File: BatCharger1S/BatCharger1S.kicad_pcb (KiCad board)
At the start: 2 copper layers, 53.7 x 25.7 mm, 58 parts, among them J1 USB_C_Receptacle, J2 01x02, J3 01x02, J4 01x02, J5 01x02, J6 Conn_01x03, J7 01x02, Q1 Si2323DS, Q2 Si2323DS, Q3 Si2323DS, Q4 Si2323DS, U1 USBLC6-2P6, U2 MAX17048G+T10, U3 MCP73833-AMI/UN, U4 TLV75533PDBV

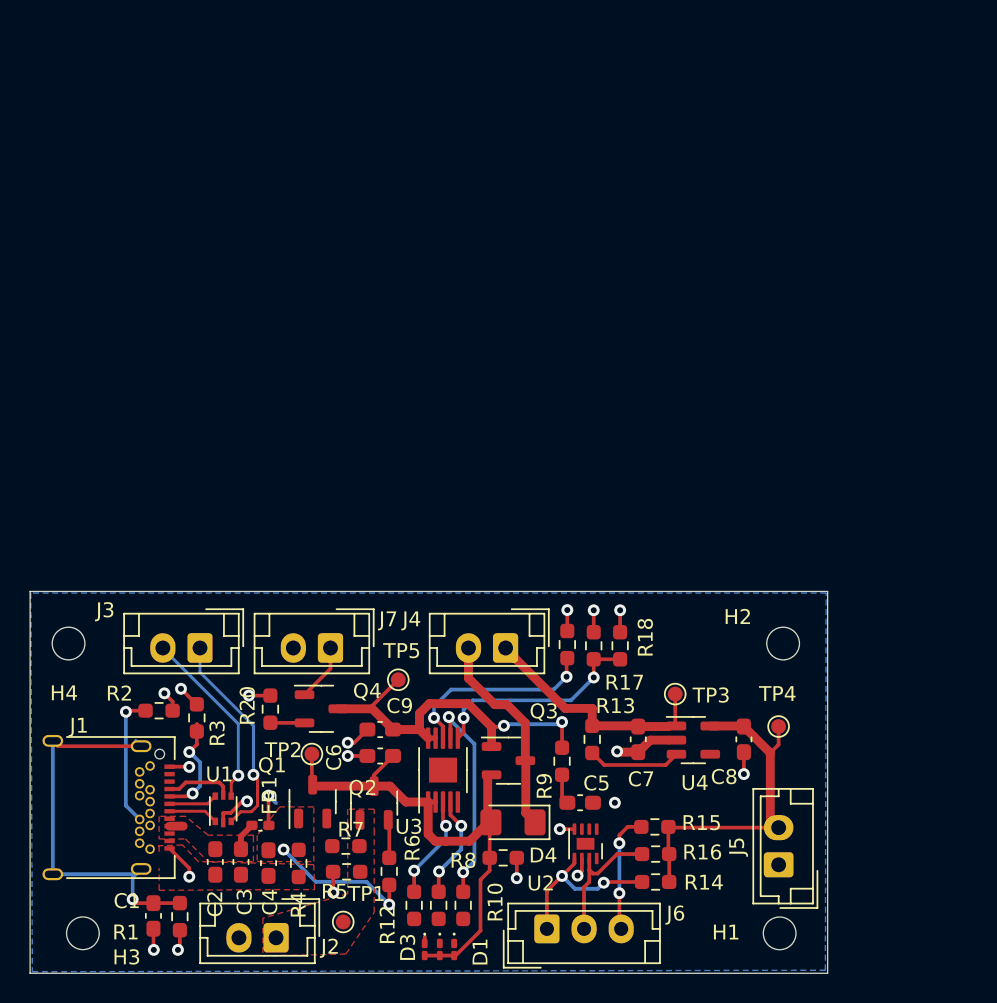
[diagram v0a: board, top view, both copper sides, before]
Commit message: v2Layout
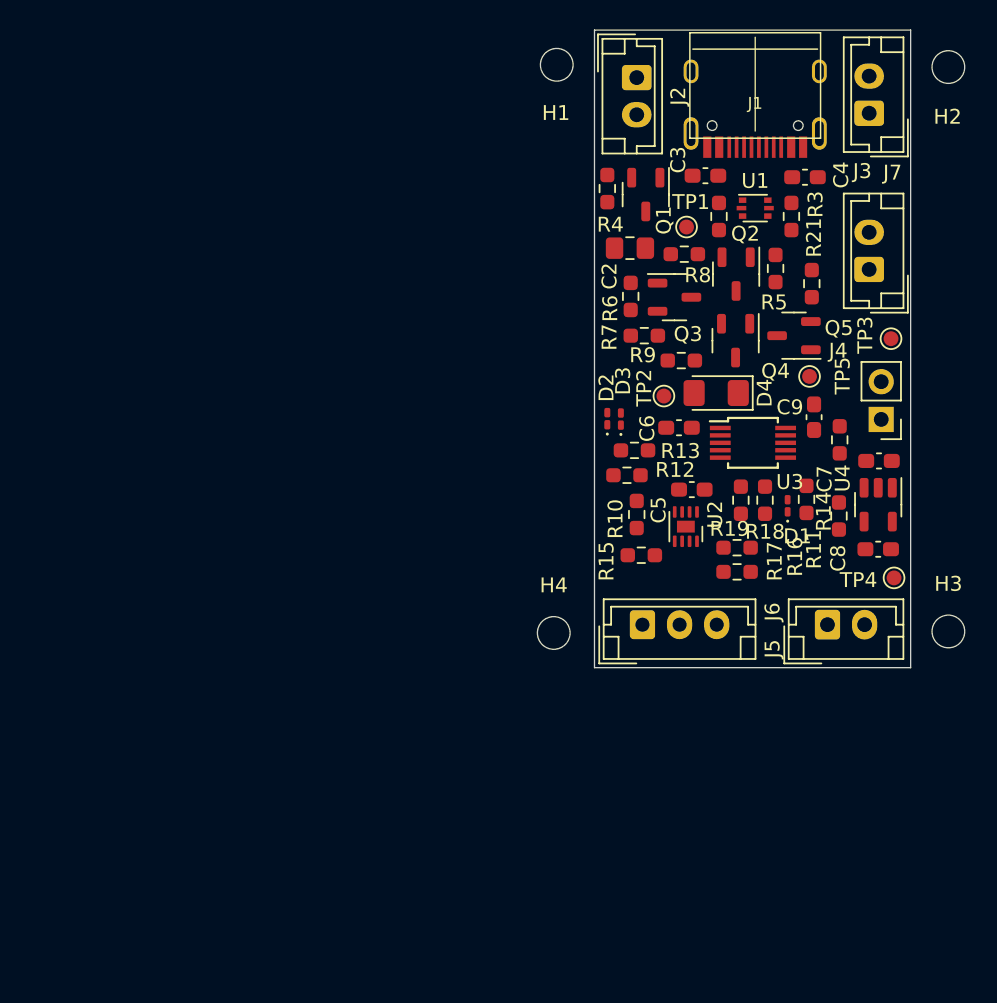
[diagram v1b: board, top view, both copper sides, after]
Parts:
- removed C1: 10u, Capacitor_SMD:C_0603_1608Metric_Pad1.08x0.95mm_HandSolder
- removed FB1: 100 @ 100MHz, Inductor_SMD:L_0402_1005Metric_Pad0.77x0.64mm_HandSolder
- removed R1: 1M, Resistor_SMD:R_0603_1608Metric_Pad0.98x0.95mm_HandSolder
- added Q5: Si2323DS, Package_TO_SOT_SMD:SOT-23-3, F.Cu at (145.6, 64.2)
- added R21: 100k, Resistor_SMD:R_0603_1608Metric_Pad0.98x0.95mm_HandSolder, F.Cu at (146.8, 60.7)
- C2: footprint Capacitor_SMD:C_0603_1608Metric_Pad1.08x0.95mm_HandSolder -> Capacitor_SMD:C_0805_2012Metric_Pad1.18x1.45mm_HandSolder
- C3: value 1u -> 10u
- J1: value USB_C_Receptacle -> TYPE-C-31-M-12; footprint Connector_USB:USB_C_Receptacle_Amphenol_12401548E4-2A -> Connector_USB:TYPE-C-31-M-12
- J4: footprint Connector_JST:JST_EH_B2B-EH-A_1x02_P2.50mm_Vertical -> Connector_PinHeader_2.54mm:PinHeader_1x02_P2.54mm_Vertical
- J5: value 01x02 -> Conn_01x03; footprint Connector_JST:JST_EH_B2B-EH-A_1x02_P2.50mm_Vertical -> Connector_JST:JST_EH_B3B-EH-A_1x03_P2.50mm_Vertical
- J6: value Conn_01x03 -> 01x02; footprint Connector_JST:JST_EH_B3B-EH-A_1x03_P2.50mm_Vertical -> Connector_JST:JST_EH_B2B-EH-A_1x02_P2.50mm_Vertical
- R10: value 1k -> 0R
- R13: value 100k -> 1k
- R14, R6: value 10k -> 100k
- R15: value 2k2 -> 10k
- R17: value 1k -> 2k2
- R19: value 10k -> 1k
- R20, R4, R8: value 100k -> 10k
- R9: value 0R -> 100k
- U3: footprint Package_SO:MSOP-10-1EP_3x3mm_P0.5mm_EP1.68x1.88mm -> Package_SO:MSOP-10_3x3mm_P0.5mm
- moved J1 66.6 mm to (143.0, 46.4), turned to 180 degrees
- moved J2 62.8 mm to (135.0, 46.8), turned to -90 degrees
- moved H3 61.7 mm to (156.0, 84.1)
- moved H1 60.4 mm to (129.6, 45.9)
- moved C4 58.6 mm to (146.4, 53.5), turned to 0 degrees
- moved J3 57.7 mm to (150.7, 49.2), turned to 90 degrees
- moved C3 55.8 mm to (139.7, 53.4), turned to 180 degrees
- moved U1 54.0 mm to (143.0, 55.6), turned to 0 degrees
- moved R3 52.4 mm to (145.4, 56.1), turned to -90 degrees
- moved TP1 52.2 mm to (138.4, 56.8)
- moved R2 50.3 mm to (140.6, 56.1), turned to -90 degrees
- moved R4 50.0 mm to (133.0, 54.3)
- moved C2 49.9 mm to (134.6, 58.3), turned to 180 degrees
- moved R5 49.8 mm to (144.4, 59.6), turned to -90 degrees
- moved Q1 46.6 mm to (135.6, 54.7), turned to -90 degrees
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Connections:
- C2 pad 1: /VBUS_IN -> +5V
- C3 pad 1: /VBUS_IN -> VBUS
- J1 pad A4: /VBUS_IN -> VBUS
- J1 pad A8: unconnected-(J1-SBU1-PadA8) -> (no net)
- J1 pad A9: /VBUS_IN -> VBUS
- J1 pad B4: /VBUS_IN -> VBUS
- J1 pad B6: /CON_USB_P -> (no net)
- J1 pad B7: /CON_USB_N -> (no net)
- J1 pad B8: unconnected-(J1-SBU2-PadB8) -> (no net)
- J1 pad B9: /VBUS_IN -> VBUS
- J1 pad S1: Net-(J1-SHIELD) -> GND
- J2 pad 1: +5V -> GND
- J2 pad 2: GND -> Net-(J2-Pin_2)
- J5 pad 1: GND -> /Alert
- J5 pad 2: +3V3 -> /SDA
- J6 pad 1: /Alert -> GND
- J6 pad 2: /SCl -> +3V3
- Q1 pad 1: VBUS -> Net-(J2-Pin_2)
- Q1 pad 3: VDC -> +5V
- Q2 pad 1: +5V -> VBUS
- Q3 pad 1: +BATT -> +5V
- Q3 pad 2: VDC -> Net-(Q3-G)
- Q3 pad 3: /pwrSwitch -> VDC
- Q4 pad 1: Net-(J7-Pin_1) -> +BATT
- Q4 pad 2: Net-(Q4-G) -> VDC
- Q4 pad 3: +BATT -> /pwrSwitch
- R10 pad 1: Net-(D1-K) -> +BATT
- R10 pad 2: Net-(U3-nPG) -> /vBatSense
- R11 pad 1: Net-(D2-K) -> Net-(D1-K)
- R11 pad 2: Net-(U3-STAT2) -> Net-(U3-nPG)
- R12 pad 1: Net-(D3-K) -> Net-(D2-K)
- R12 pad 2: Net-(U3-STAT1) -> Net-(U3-STAT2)
- R13 pad 1: VCC -> Net-(D3-K)
- R13 pad 2: Net-(U4-EN) -> Net-(U3-STAT1)
- R14 pad 1: +3V3 -> VCC
- R14 pad 2: /Alert -> Net-(U4-EN)
- R15 pad 2: /SDA -> /Alert
- R16 pad 2: /SCl -> /SDA
- R17 pad 1: Net-(U3-PROG) -> +3V3
- R17 pad 2: GND -> /SCl
- R19 pad 1: Net-(U3-THERM) -> Net-(U3-PROG)
- R20 pad 1: GND -> Net-(U3-THERM)
- R20 pad 2: Net-(Q4-G) -> GND
- R4 pad 1: VBUS -> Net-(Q1-G)
- R5 pad 1: GND -> VBUS
- R5 pad 2: +5V -> GND
- R6 pad 1: VBUS -> GND
- R6 pad 2: Net-(Q2-G) -> +5V
- R7 pad 1: Net-(Q1-G) -> VBUS
- R7 pad 2: +5V -> Net-(Q3-G)
- R8 pad 1: GND -> Net-(Q2-G)
- R8 pad 2: VDC -> +5V
- R9 pad 1: +BATT -> GND
- R9 pad 2: /vBatSense -> VDC
- U1 pad 5: /VBUS_IN -> VBUS
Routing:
- net VDC: track 36.0 -> 0.00 mm
- net GND: track 31.1 -> 0.00 mm, vias 20 -> 0
- net Net-(J1-SHIELD): track 26.7 -> 0.00 mm, vias 1 -> 0
- net +BATT: track 25.2 -> 0.00 mm, vias 2 -> 0
- net +3V3: track 23.5 -> 0.00 mm
- net VCC: track 16.0 -> 0.00 mm
- net Net-(U3-PROG): track 14.8 -> 0.00 mm, vias 2 -> 0
- net /USB_N: track 14.3 -> 0.00 mm, vias 1 -> 0
- net Net-(U3-nPG): track 14.3 -> 0.00 mm, vias 2 -> 0
- net /pwrSwitch: track 14.3 -> 0.00 mm
- net Net-(U3-THERM): track 13.6 -> 0.00 mm, vias 2 -> 0
- net VBUS: track 12.8 -> 0.00 mm, vias 3 -> 0
- net /USB_P: track 12.2 -> 0.00 mm, vias 1 -> 0
- net /Alert: track 11.4 -> 0.00 mm, vias 2 -> 0
- net /SCl: track 9.83 -> 0.00 mm
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- removed copper zone on F.Cu, net +5V
- removed copper zone on F.Cu, net /VBUS_IN
- removed copper zone on B.Cu, net GND
- removed copper zone on F.Cu, net GND
- removed copper zone on F.Cu, net VBUS
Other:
- board size 53.7 x 25.7 mm -> 21.3 x 42.9 mm
